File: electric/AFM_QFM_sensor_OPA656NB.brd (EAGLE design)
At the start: 37.8 x 48.2 mm, 22 parts, among them J4 USBR-A-S-S-O-TH, U2 AD8676ARMZ, U3 AD8675ARMZ-REEL, U4 OPA656U

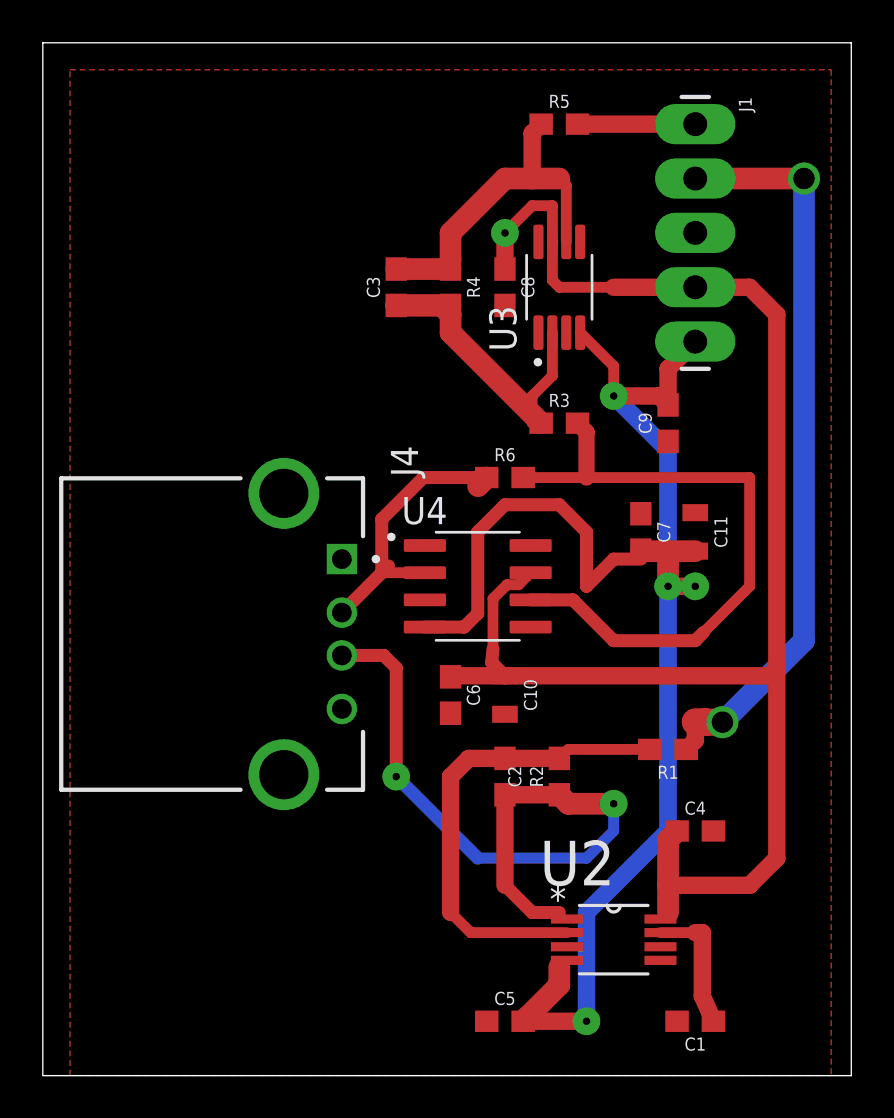
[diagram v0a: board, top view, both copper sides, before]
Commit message: newer electroincs
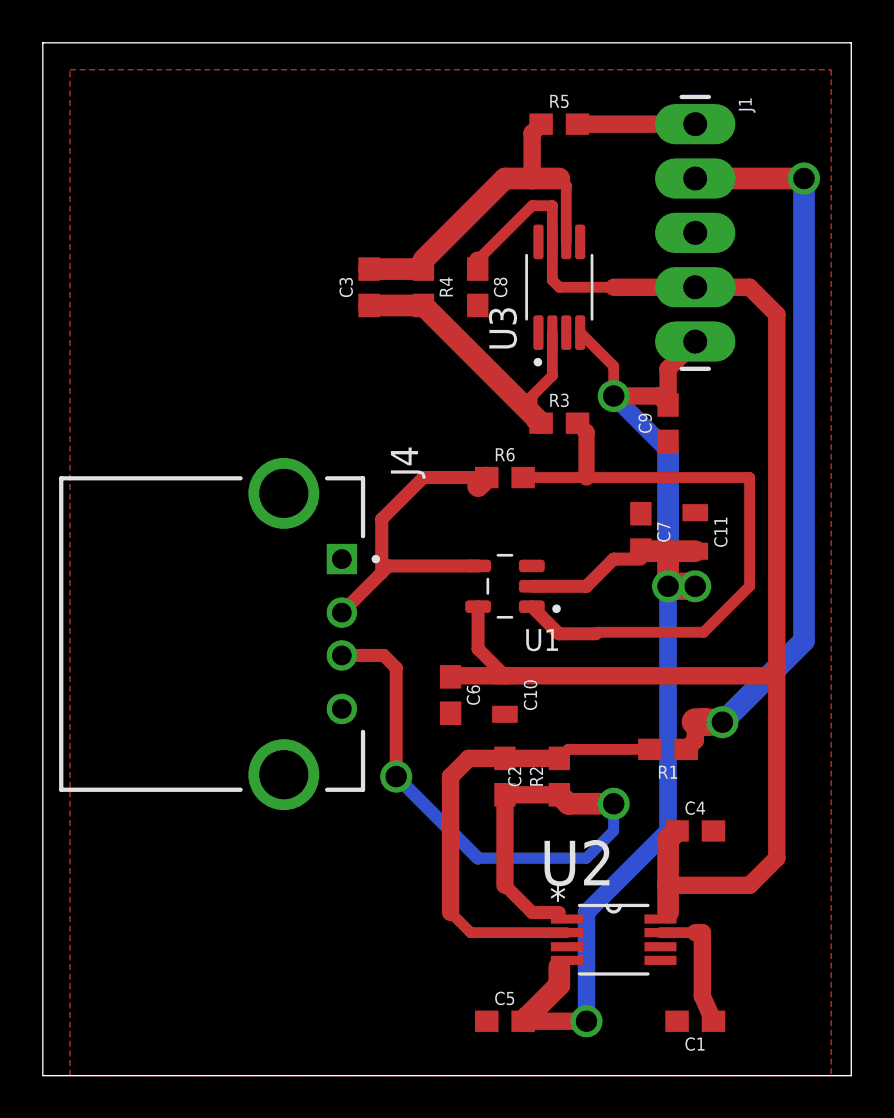
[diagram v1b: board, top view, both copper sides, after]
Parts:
- removed U4: OPA656U, OPA656U:SOIC127P599X175-8N
- added U1: OPA656NB/250, OPA656NB_250:SOT95P280X145-5N
- moved C3 1.27 mm to (14.0, 35.6)
- moved C8 1.27 mm to (19.1, 35.6)
- moved R4 1.27 mm to (16.5, 35.6)
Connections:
- net AGND: now also U1.3; no longer U4.3
- net N$3: now also U1.4; no longer U4.2
- net OPA_OUT: now also U1.1; no longer U4.6
- net V+: now also U1.5; no longer U4.7
- net V-: now also U1.2; no longer U4.4
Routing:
- net V-: track 71.5 -> 58.8 mm
- net OPA_OUT: track 47.2 -> 44.9 mm
- net N$3: track 13.9 -> 16.1 mm
- net V+: track 76.1 -> 74.3 mm, vias 1 -> 0
- net N$8: track 15.8 -> 16.3 mm
